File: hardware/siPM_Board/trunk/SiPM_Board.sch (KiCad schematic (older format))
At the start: 25 parts, among them J1 Conn_02x34_Odd_Even, J2 Conn_02x34_Odd_Even, U1 LM94021, U2 S14161-6050HS-04, U3 S14161-6050HS-04, U4 S14161-6050HS-04, U5 S14161-6050HS-04

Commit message: Layout Needs Editing
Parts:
- C1, C10, C11, C12, C13, C14, C15, C16, C17, C18, C2, C3, C4, C5, C6, C7, C8, C9: footprint Capacitor_SMD:C_1206_3216Metric_Pad1.33x1.80mm_HandSolder -> Capacitor_SMD:C_0603_1608Metric_Pad1.08x0.95mm_HandSolder; Item Cost $0.85 -> $0.12; MFN C3216C0G2A104J160AC -> 0603B104K101CT; Supplier P/N 445-172677-1-ND -> 1292-1392-1-ND

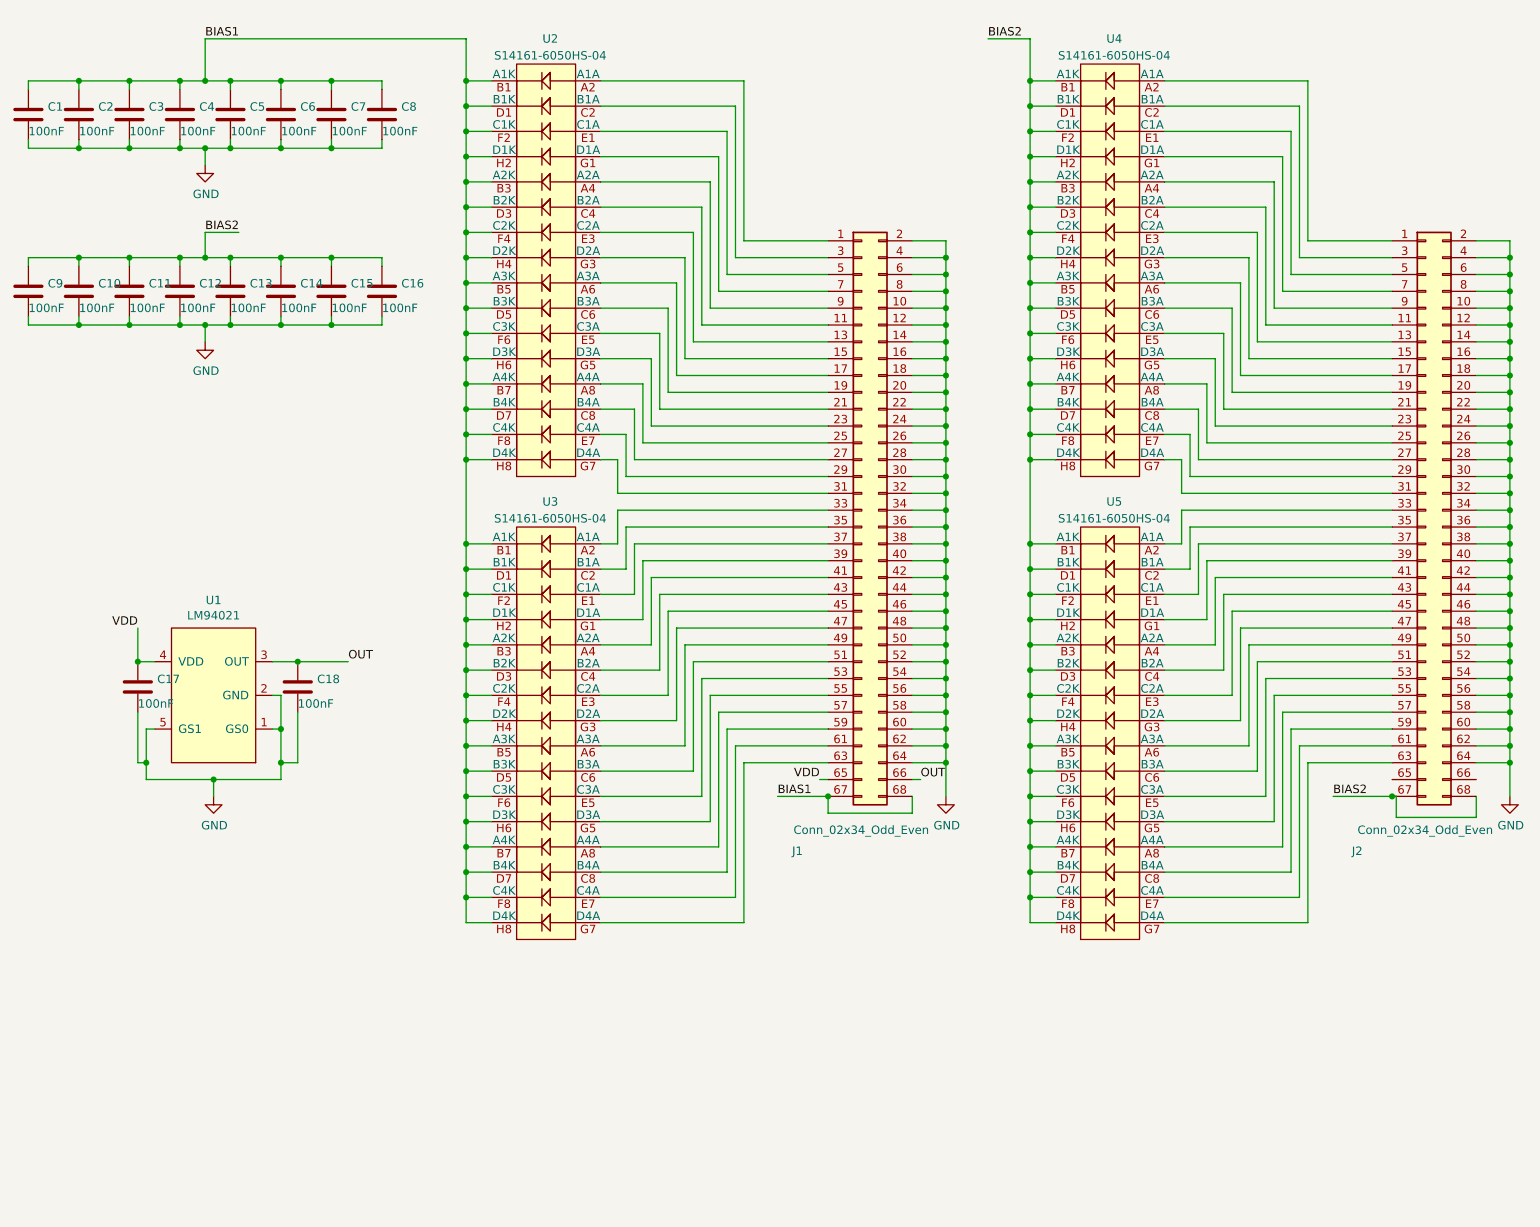
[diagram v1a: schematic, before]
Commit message: Schematic changes made
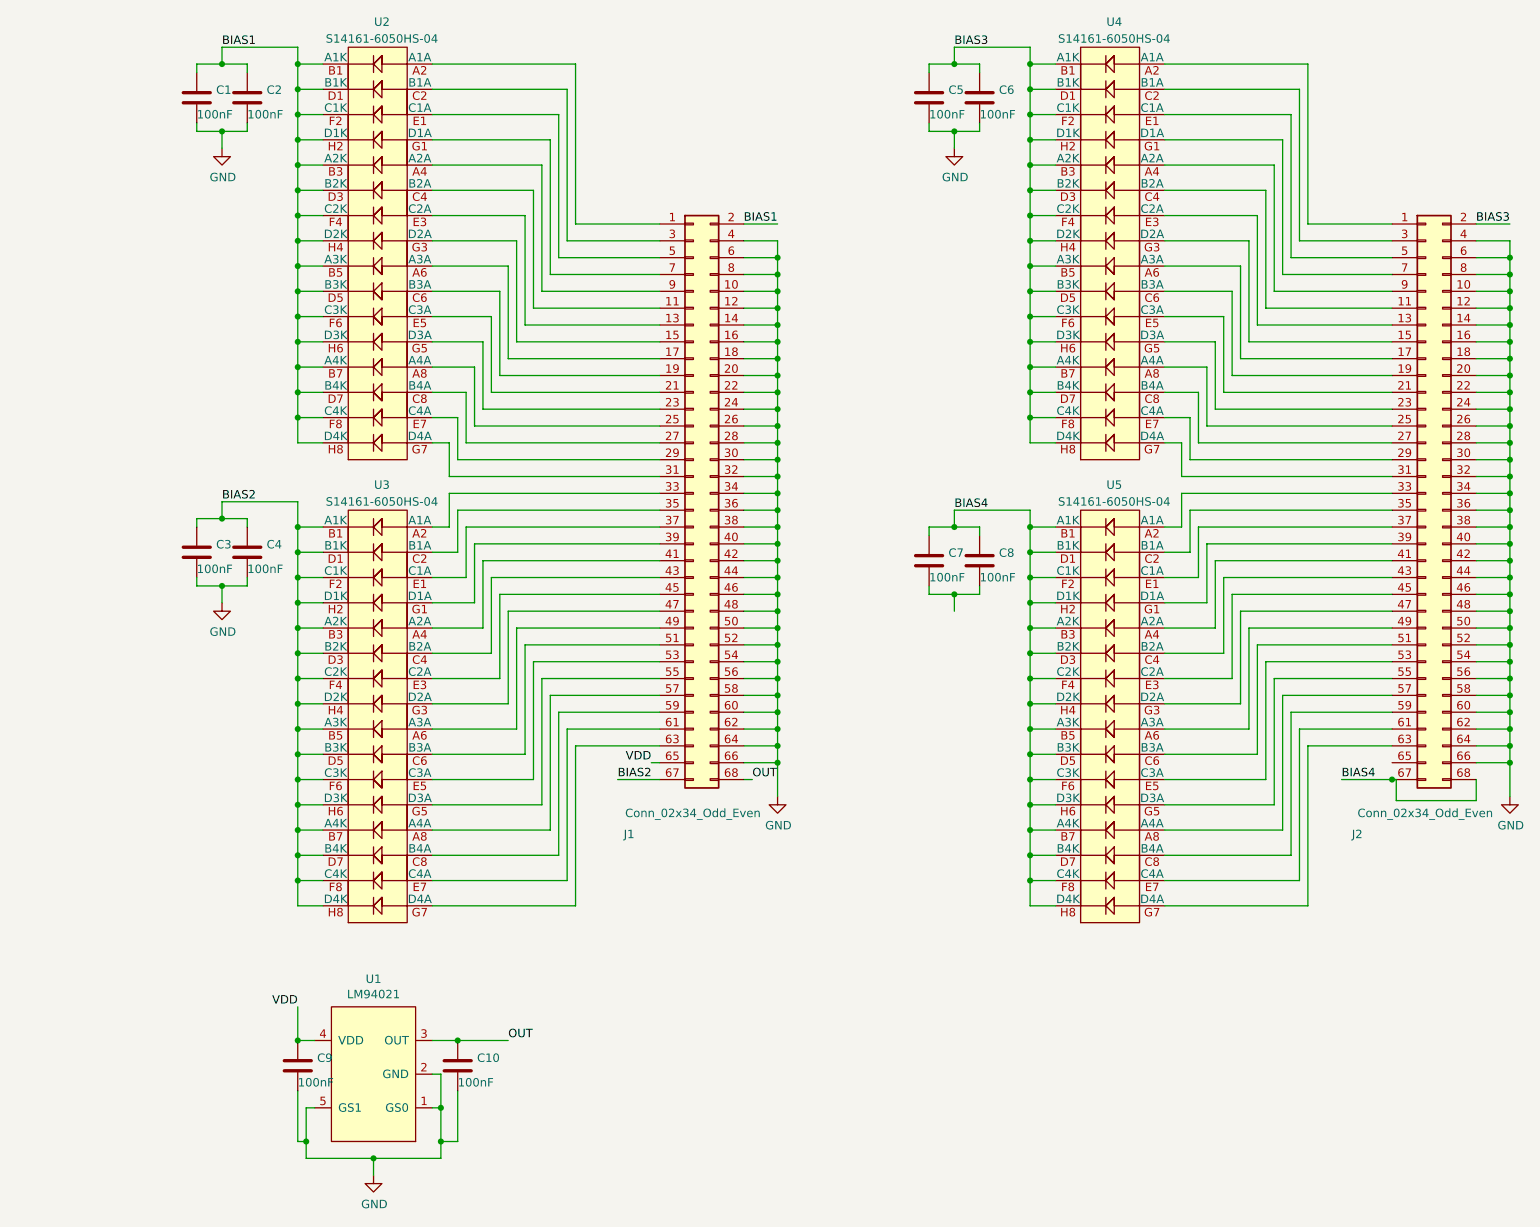
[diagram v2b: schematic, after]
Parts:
- removed C10, C11, C14, C15, C16, C5, C6, C9: 100nF, Capacitor_SMD:C_0603_1608Metric_Pad1.08x0.95mm_HandSolder, symbol Device:C
- renumbered C18 to C10, C12 to C5, C13 to C6, C17 to C9
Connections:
- net BIAS1: now also J1.2 (Pin_2); no longer C3.1, C4.1, C7.1, C8.1, J1.67 (Pin_67), J1.68 (Pin_68), U3.B1 (A1K), U3.B3 (A2K), U3.B5 (A3K), U3.B7 (A4K), U3.D1 (B1K), U3.D3 (B2K), U3.D5 (B3K), U3.D7 (B4K), U3.F2 (C1K), U3.F4 (C2K), U3.F6 (C3K), U3.F8 (C4K), U3.H2 (D1K), U3.H4 (D2K), U3.H6 (D3K), U3.H8 (D4K)
- net BIAS2: now also C3.1, C4.1, J1.67 (Pin_67), U3.B1 (A1K), U3.B3 (A2K), U3.B5 (A3K), U3.B7 (A4K), U3.D1 (B1K), U3.D3 (B2K), U3.D5 (B3K), U3.D7 (B4K), U3.F2 (C1K), U3.F4 (C2K), U3.F6 (C3K), U3.F8 (C4K), U3.H2 (D1K), U3.H4 (D2K), U3.H6 (D3K), U3.H8 (D4K); no longer C5.1, C6.1, J2.67 (Pin_67), J2.68 (Pin_68), U4.B1 (A1K), U4.B3 (A2K), U4.B5 (A3K), U4.B7 (A4K), U4.D1 (B1K), U4.D3 (B2K), U4.D5 (B3K), U4.D7 (B4K), U4.F2 (C1K), U4.F4 (C2K), U4.F6 (C3K), U4.F8 (C4K), U4.H2 (D1K), U4.H4 (D2K), U4.H6 (D3K), U4.H8 (D4K), U5.B1 (A1K), U5.B3 (A2K), U5.B5 (A3K), U5.B7 (A4K), U5.D1 (B1K), U5.D3 (B2K), U5.D5 (B3K), U5.D7 (B4K), U5.F2 (C1K), U5.F4 (C2K), U5.F6 (C3K), U5.F8 (C4K), U5.H2 (D1K), U5.H4 (D2K), U5.H6 (D3K), U5.H8 (D4K)
- net GND: now also J1.66 (Pin_66), J2.66 (Pin_66); no longer C7.2, C8.2, J1.2 (Pin_2), J2.2 (Pin_2)
- net OUT: now also J1.68 (Pin_68); no longer J1.66 (Pin_66)
- new net: C7.2, C8.2
- new net BIAS3: C5.1, C6.1, J2.2 (Pin_2), U4.B1 (A1K), U4.B3 (A2K), U4.B5 (A3K), U4.B7 (A4K), U4.D1 (B1K), U4.D3 (B2K), U4.D5 (B3K), U4.D7 (B4K), U4.F2 (C1K), U4.F4 (C2K), U4.F6 (C3K), U4.F8 (C4K), U4.H2 (D1K), U4.H4 (D2K), U4.H6 (D3K), U4.H8 (D4K)
- new net BIAS4: C7.1, C8.1, J2.67 (Pin_67), J2.68 (Pin_68), U5.B1 (A1K), U5.B3 (A2K), U5.B5 (A3K), U5.B7 (A4K), U5.D1 (B1K), U5.D3 (B2K), U5.D5 (B3K), U5.D7 (B4K), U5.F2 (C1K), U5.F4 (C2K), U5.F6 (C3K), U5.F8 (C4K), U5.H2 (D1K), U5.H4 (D2K), U5.H6 (D3K), U5.H8 (D4K)
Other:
- moved on the sheet: C10, C5, C6, C9, J1, J2, U1, U2, U3, U4, U5
